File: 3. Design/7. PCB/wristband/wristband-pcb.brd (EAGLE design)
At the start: 27.5 x 36.3 mm, 44 parts, among them IC1 STM32F051K8T6, Y2 FA-20H_16.0000MF12Z-AC3, Y3 FA-20H_16.0000MF12Z-AC3

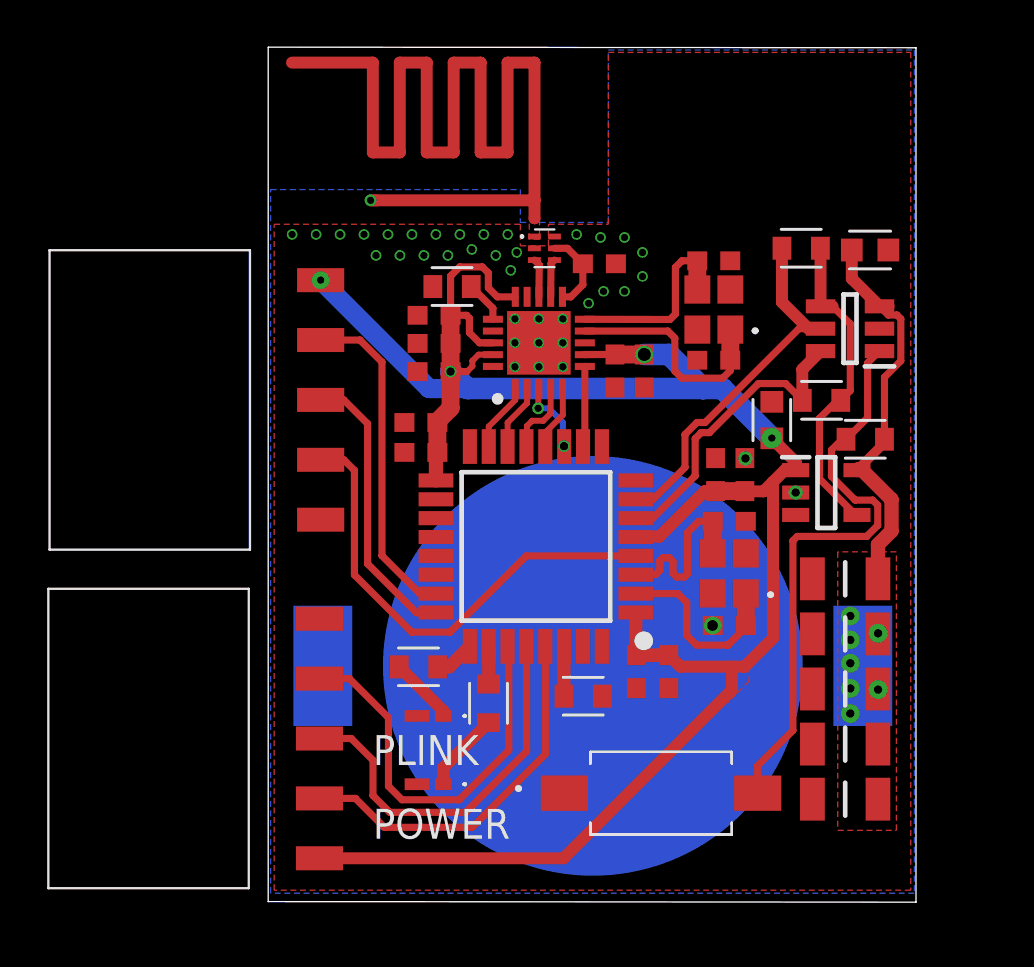
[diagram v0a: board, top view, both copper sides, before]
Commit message: ADD|UPDT: Exported new and corrected old 3D models, 2D models and technical drawings of all  PCBs
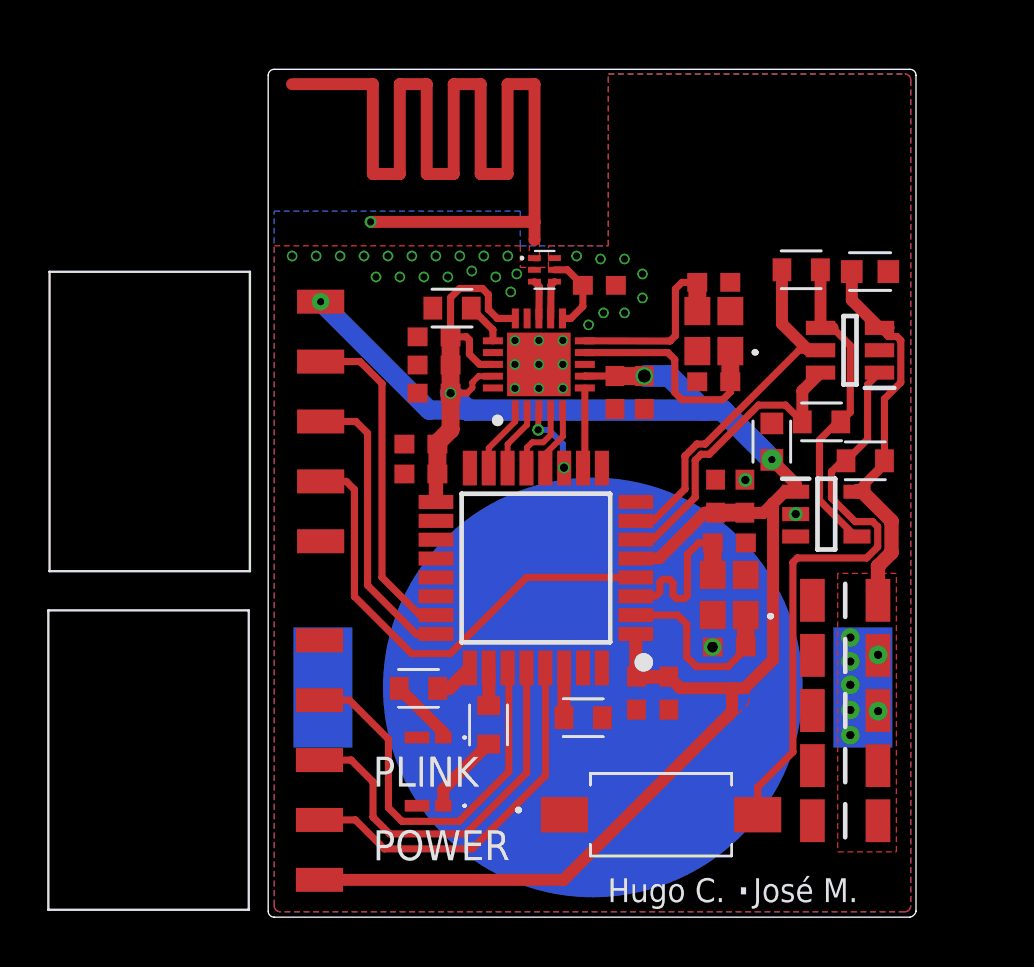
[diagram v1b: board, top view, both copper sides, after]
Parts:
- moved ANT1 0.91 mm to (11.7, 27.5)
- moved BATT_HLD 0.91 mm to (13.8, 9.74)
- moved C1 0.91 mm to (21.4, 20.2)
- moved C10 0.91 mm to (24.5, 8.76)
- moved C11 0.91 mm to (24.5, 13.4)
- moved C12 0.91 mm to (24.5, 11.1)
- moved C14 0.91 mm to (24.5, 6.43)
- moved C15 0.91 mm to (18.9, 22.7)
- moved C16 0.91 mm to (18.9, 26.9)
- moved C17 0.91 mm to (19.6, 11.5)
- moved C18 0.91 mm to (19.6, 15.9)
- moved C19 0.91 mm to (6.48, 18.8)
- moved C2 0.91 mm to (25.5, 27.4)
- moved C20 0.91 mm to (17.0, 9.50)
- moved C21 0.91 mm to (15.6, 9.50)
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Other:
- board size 27.5 x 36.3 mm -> 27.5 x 36 mm
- board text added: "."
- board text added: "Hugo C. José M."

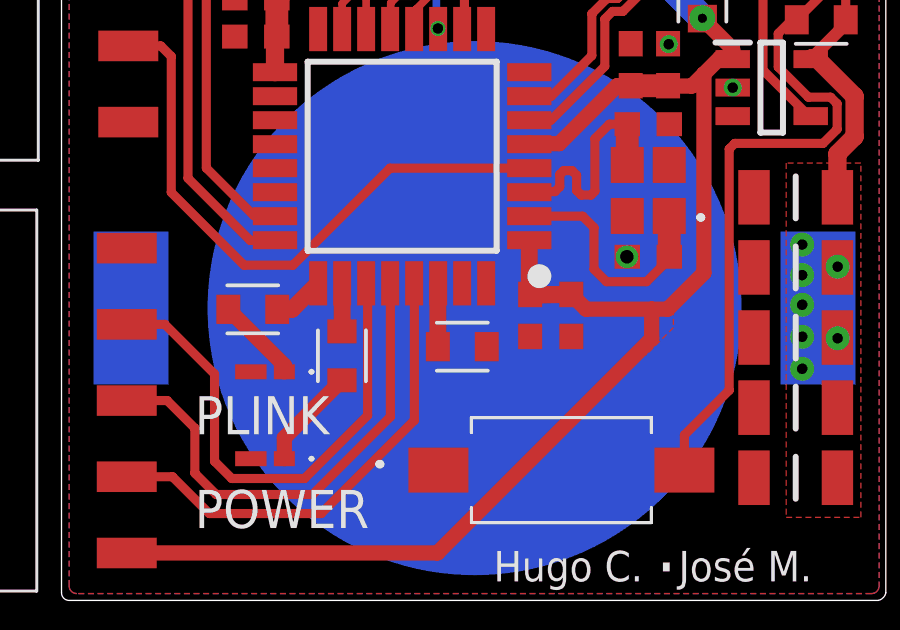
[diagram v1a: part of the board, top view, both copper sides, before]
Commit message: ADD: pb-switch and wristband CAM files
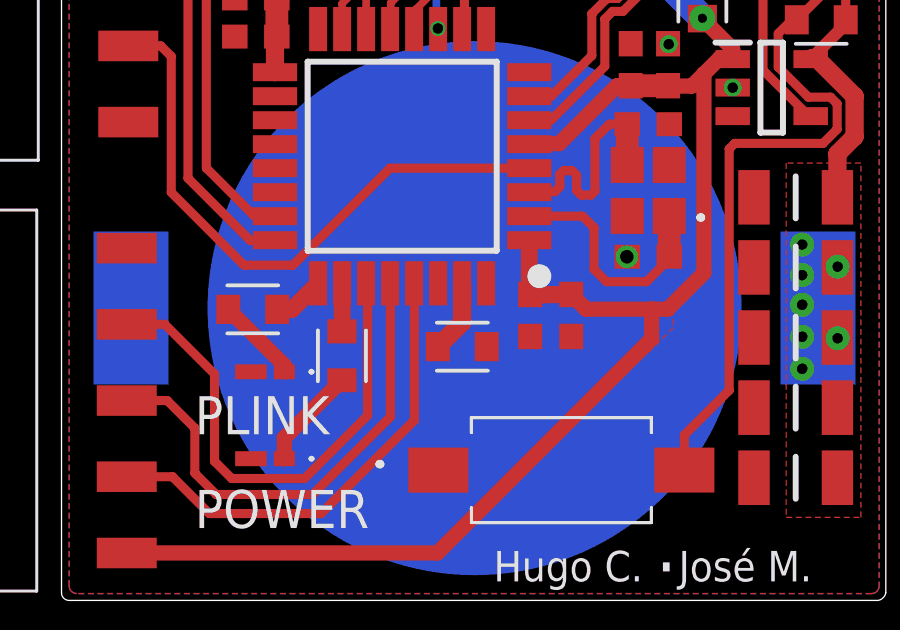
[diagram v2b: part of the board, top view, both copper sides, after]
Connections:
- net N$4: now also IC1.31; no longer IC1.30
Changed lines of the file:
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@@
 <signal name="N$4">
 <contactref element="R7" pad="1"/>
-<contactref element="IC1" pad="30"/>
-<wire x1="12.5538" y1="10.5702" x2="12.5452" y2="10.5616" width="0.5588" layer="1"/>
-<wire x1="12.5452" y1="10.5616" x2="12.5452" y2="8.4582" width="0.5588" layer="1"/>
+<contactref element="IC1" pad="31"/>
+<wire x1="13.3538" y1="10.5702" x2="13.3538" y2="9.2668" width="0.6096" layer="1"/>
+<wire x1="13.3538" y1="9.2668" x2="12.5452" y2="8.4582" width="0.6096" layer="1"/>
 </signal>
 <signal name="FLG">

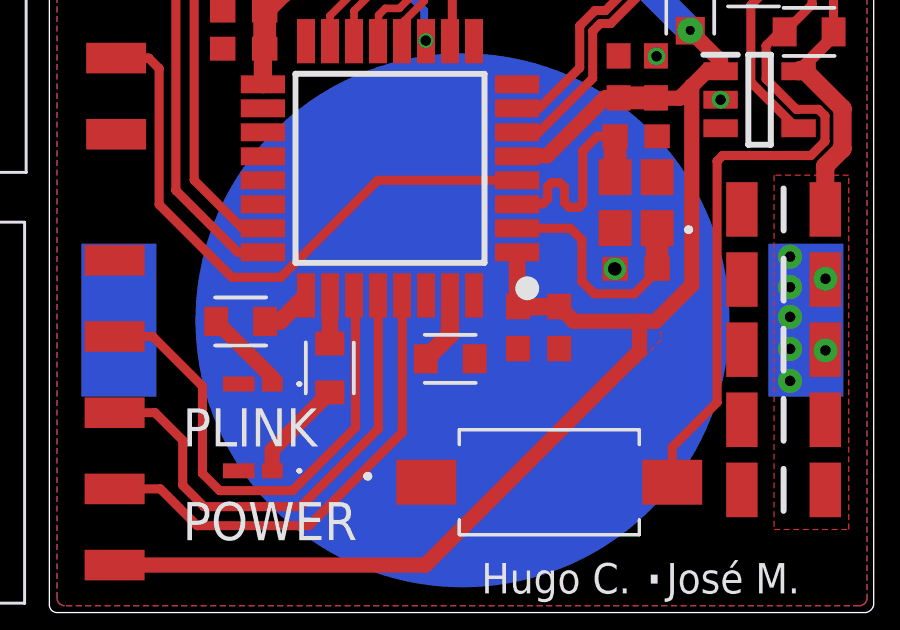
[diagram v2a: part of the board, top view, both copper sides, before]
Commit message: Project at the time of delivery
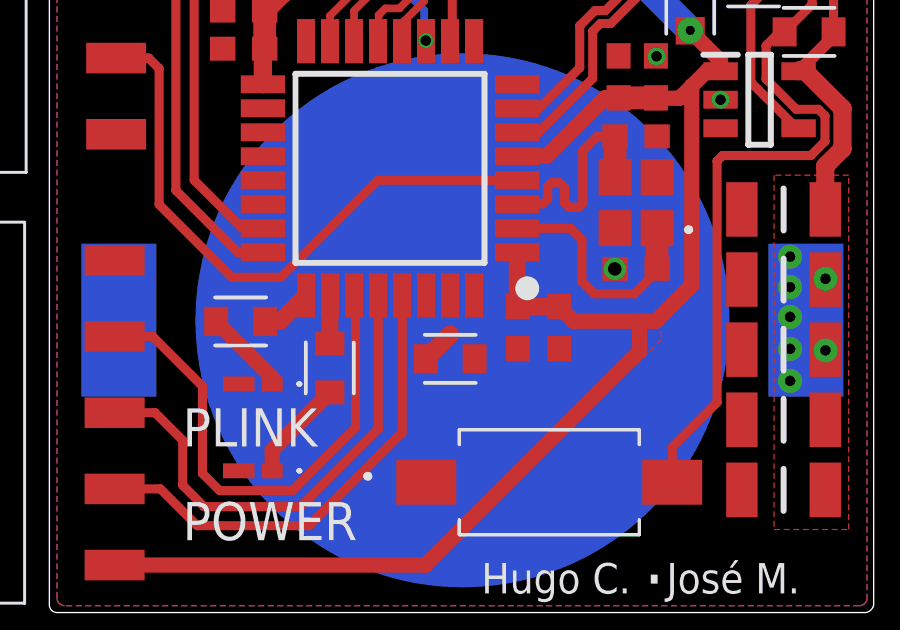
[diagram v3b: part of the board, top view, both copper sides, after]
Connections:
- net N$4: now also IC1.30; no longer IC1.31
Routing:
- net N$4: track 2.45 -> 1.14 mm
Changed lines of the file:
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@@
 <drawing>
 <settings>
-<setting alwaysvectorfont="yes"/>
+<setting alwaysvectorfont="no"/>
 <setting verticaltext="up"/>
 </settings>
@@
 </layers>
 <board>
-<fusionsync huburn="a.YnVzaW5lc3M6YWx1bm9zNjU4" projecturn="a.YnVzaW5lc3M6YWx1bm9zNjU4I0QyMDIwMTEyNjM1NzA0MDM1MQ" f3durn="urn:adsk.wipprod:dm.lineage:bKpgsLsdQMqy66-_QmCFMA" pcbguid="" lastpulledtime="2020-12-20T21:33:40Z" lastsyncedchangeguid="" latestrevisionid="9daa5ef3-dd75-4898-81f4-dd43f1275c59" lastsyncedrevisionid="9daa5ef3-dd75-4898-81f4-dd43f1275c59" lastboardhashguid="ac83953b-309a-8dae-37b7-7914f2571517" lastpushedtime="2020-12-20T22:28:16Z" linktopcb3d="true"/>
+<fusionsync huburn="a.YnVzaW5lc3M6YWx1bm9zNjU4" projecturn="a.YnVzaW5lc3M6YWx1bm9zNjU4I0QyMDIwMTEyNjM1NzA0MDM1MQ" f3durn="urn:adsk.wipprod:dm.lineage:bKpgsLsdQMqy66-_QmCFMA" pcbguid="" lastpulledtime="2020-12-20T21:33:40Z" lastsyncedchangeguid="" latestrevisionid="9daa5ef3-dd75-4898-81f4-dd43f1275c59" lastsyncedrevisionid="9daa5ef3-dd75-4898-81f4-dd43f1275c59" lastboardhashguid="ac83953b-309a-8dae-37b7-7914f2571517" lastpushedtime="2020-12-20T22:28:16Z" linktopcb3d="false"/>
 <plain>
 <text x="4.445" y="2.413" size="1.27" layer="21" font="vector" ratio="16">POWER</text>
@@
 <signal name="N$4">
 <contactref element="R7" pad="1"/>
-<contactref element="IC1" pad="31"/>
-<wire x1="13.3538" y1="10.5702" x2="13.3538" y2="9.2668" width="0.6096" layer="1"/>
 <wire x1="13.3538" y1="9.2668" x2="12.5452" y2="8.4582" width="0.6096" layer="1"/>
+<contactref element="IC1" pad="30"/>
+<wire x1="13.3538" y1="9.2668" x2="12.5538" y2="10.5702" width="0" layer="19" extent="1-1"/>
 </signal>
 <signal name="FLG">
